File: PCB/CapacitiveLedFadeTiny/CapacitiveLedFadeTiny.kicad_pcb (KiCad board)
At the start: 2 copper layers, 36.3 x 36.3 mm, 7 parts, among them J1 Bus In, J2 Bus Out, J3 LEDs, J4 Antenna, U1 ATTINY85-20SU

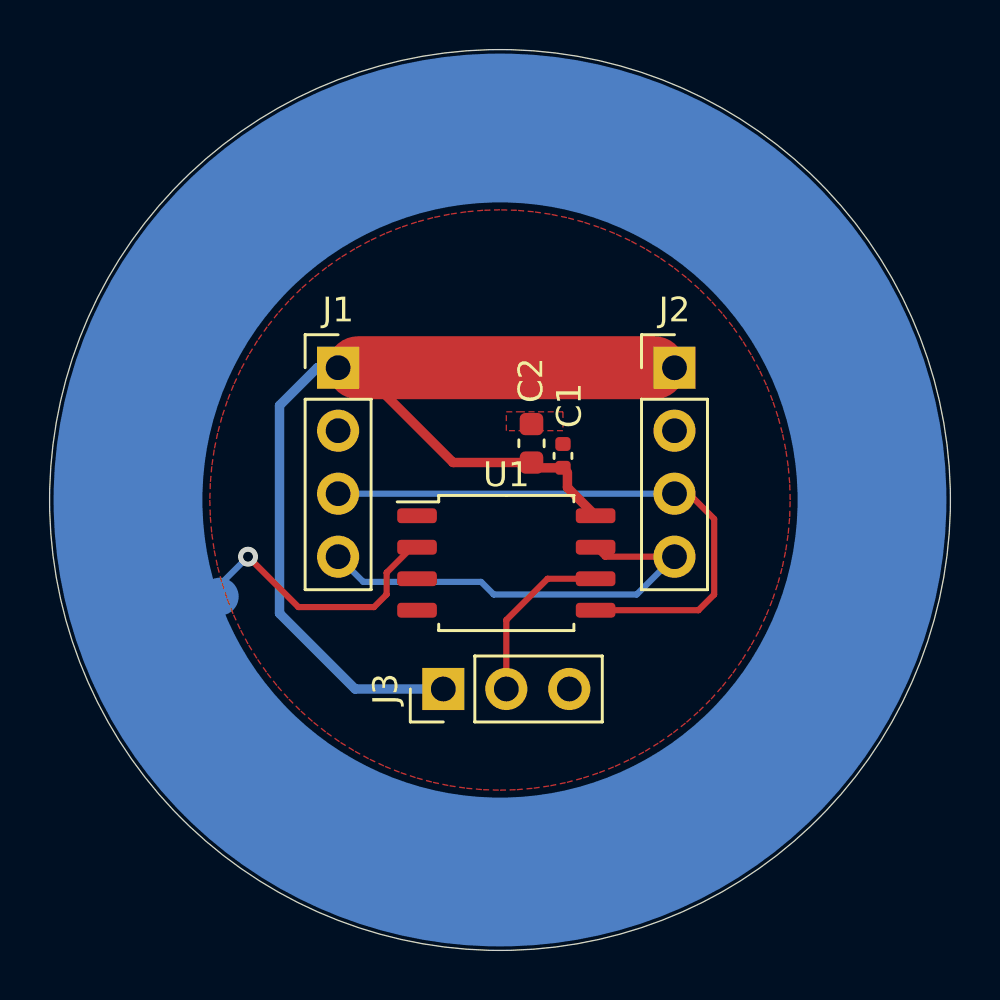
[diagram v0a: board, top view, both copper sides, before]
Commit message: v2 of I2C board
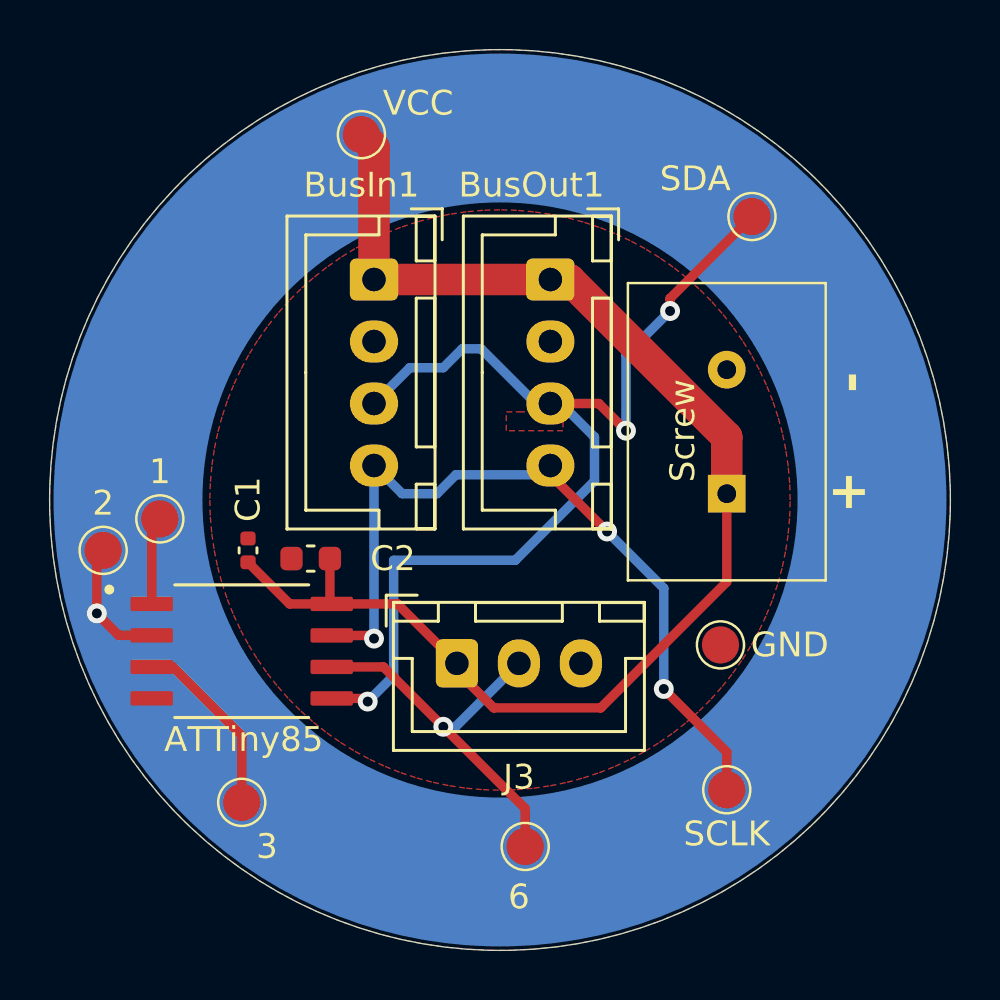
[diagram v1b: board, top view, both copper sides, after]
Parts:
- added 1: 1, Library:TestPoint_Pad_1.5mm_circular, F.Cu at (115.3, 97.3)
- added 2: 2, Library:TestPoint_Pad_1.5mm_circular, F.Cu at (113.0, 98.6)
- added 3: 3, Library:TestPoint_Pad_1.5mm_circular, F.Cu at (118.6, 108.7)
- added 6: 6, Library:TestPoint_Pad_1.5mm_circular, F.Cu at (130.0, 110.5)
- added GND: GND, Library:TestPoint_Pad_1.5mm_circular, F.Cu at (137.9, 102.4)
- added SCLK: SCLK, Library:TestPoint_Pad_1.5mm_circular, F.Cu at (138.2, 108.2)
- added SDA: SDA, Library:TestPoint_Pad_1.5mm_circular, F.Cu at (139.2, 85.1)
- added Screw: Power Inject, Library:SCREW_TERMINAL_5mm_01x02, F.Cu at (138.2, 93.8)
- added VCC: VCC, Library:TestPoint_Pad_1.5mm_circular, F.Cu at (123.4, 81.8)
- ATTiny85: renamed from U1; footprint Package_SO:SOIC-8_5.23x5.23mm_P1.27mm -> ATTINY85-20SFR:SOIC127P798X216-8N
- BusIn1: renamed from J1; footprint Connector_PinHeader_2.54mm:PinHeader_1x04_P2.54mm_Vertical -> Connector_JST:JST_XH_B4B-XH-A_1x04_P2.50mm_Vertical
- BusOut1: renamed from J2; footprint Connector_PinHeader_2.54mm:PinHeader_1x04_P2.54mm_Vertical -> Connector_JST:JST_XH_B4B-XH-A_1x04_P2.50mm_Vertical
- J3: footprint Connector_PinHeader_2.54mm:PinHeader_1x03_P2.54mm_Vertical -> Connector_JST:JST_XH_B3B-XH-A_1x03_P2.50mm_Vertical
- moved C1 13.3 mm to (118.9, 98.6)
- moved ATTiny85 11.2 mm to (118.6, 102.6)
- moved C2 10.0 mm to (121.4, 98.9), turned to 180 degrees
- moved BusOut1 6.14 mm to (131.1, 87.6), turned to -90 degrees
- moved BusIn1 3.84 mm to (124.0, 87.6), turned to -90 degrees
- moved J3 1.17 mm to (127.3, 103.1), turned to 0 degrees
- turned J4 to 0 degrees
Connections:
- net Net-(J3-Pin_2) renamed /6
- net Net-(J4-Pin_1) renamed /2
- ATTiny85 pad 1: unconnected-(U1-PB5-Pad1) -> /1
- ATTiny85 pad 3: unconnected-(U1-PB4-Pad3) -> /3
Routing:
- net /SDA: track 23.7 -> 44.4 mm, vias 0 -> 3
- net /SCLK: track 17.4 -> 32.8 mm, vias 0 -> 3
- net VCC: track 43.6 -> 54.6 mm
- net /6: track 7.07 -> 15.8 mm, vias 0 -> 1
- net /3: track 0.00 -> 7.47 mm
- net /1: track 0.00 -> 3.56 mm
- net /2: track 11.1 -> 12.8 mm
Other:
- board text added: "+"
- board text added: "-"
